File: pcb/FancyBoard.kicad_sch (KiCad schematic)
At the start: 179 parts, among them J1 Conn_01x02_Socket, SW1 SW_Push_45deg, SW10 SW_Push_45deg, SW11 SW_Push_45deg, SW12 SW_Push_45deg, SW13 SW_Push_45deg, SW14 SW_Push_45deg, SW15 SW_Push_45deg, SW16 SW_Push_45deg, SW17 SW_Push_45deg, SW18 SW_Push_45deg, SW19 SW_Push_45deg, SW2 SW_Push_45deg, SW20 SW_Push_45deg, SW21 SW_Push_45deg, SW22 SW_Push_45deg, SW23 SW_Push_45deg, SW24 SW_Push_45deg, SW25 SW_Push_45deg, SW26 SW_Push_45deg, SW27 SW_Push_45deg, SW28 SW_Push_45deg, SW29 SW_Push_45deg, SW3 SW_Push_45deg, SW30 SW_Push_45deg, SW31 SW_Push_45deg, SW32 SW_Push_45deg, SW33 SW_Push_45deg, SW34 SW_Push_45deg, SW35 SW_Push_45deg, SW36 SW_Push_45deg, SW37 SW_Push_45deg, SW38 SW_Push_45deg, SW39 SW_Push_45deg, SW4 SW_Push_45deg, SW40 SW_Push_45deg, SW41 SW_Push_45deg, SW42 SW_Push_45deg, SW43 SW_Push_45deg, SW44 SW_Push_45deg, SW45 SW_Push_45deg, SW46 SW_Push_45deg, SW47 SW_Push_45deg, SW48 SW_Push_45deg, SW49 SW_Push_45deg, SW5 SW_Push_45deg, SW50 SW_Push_45deg, SW51 SW_Push_45deg, SW52 SW_Push_45deg, SW53 SW_Push_45deg, SW54 SW_Push_45deg, SW55 SW_Push_45deg, SW56 SW_Push_45deg, SW57 SW_Push_45deg, SW58 SW_Push_45deg, SW59 SW_Push_45deg, SW6 SW_Push_45deg, SW60 SW_Push_45deg, SW61 SW_Push_45deg, SW62 SW_Push_45deg, SW63 SW_Push_45deg, SW64 SW_Push_45deg, SW65 SW_Push_45deg, SW66 SW_Push_45deg, SW67 SW_Push_45deg, SW68 SW_Push_45deg, SW69 SW_Push_45deg, SW7 SW_Push_45deg, SW70 SW_Push_45deg, SW71 SW_Push_45deg, SW72 SW_Push_45deg, SW73 SW_Push_45deg, SW74 SW_Push_45deg, SW75 SW_Push_45deg, SW76 SW_Push_45deg, SW77 SW_Push_45deg, SW78 SW_Push_45deg, SW8 SW_Push_45deg, SW9 SW_Push_45deg, SW93 RotaryEncoder_Switch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

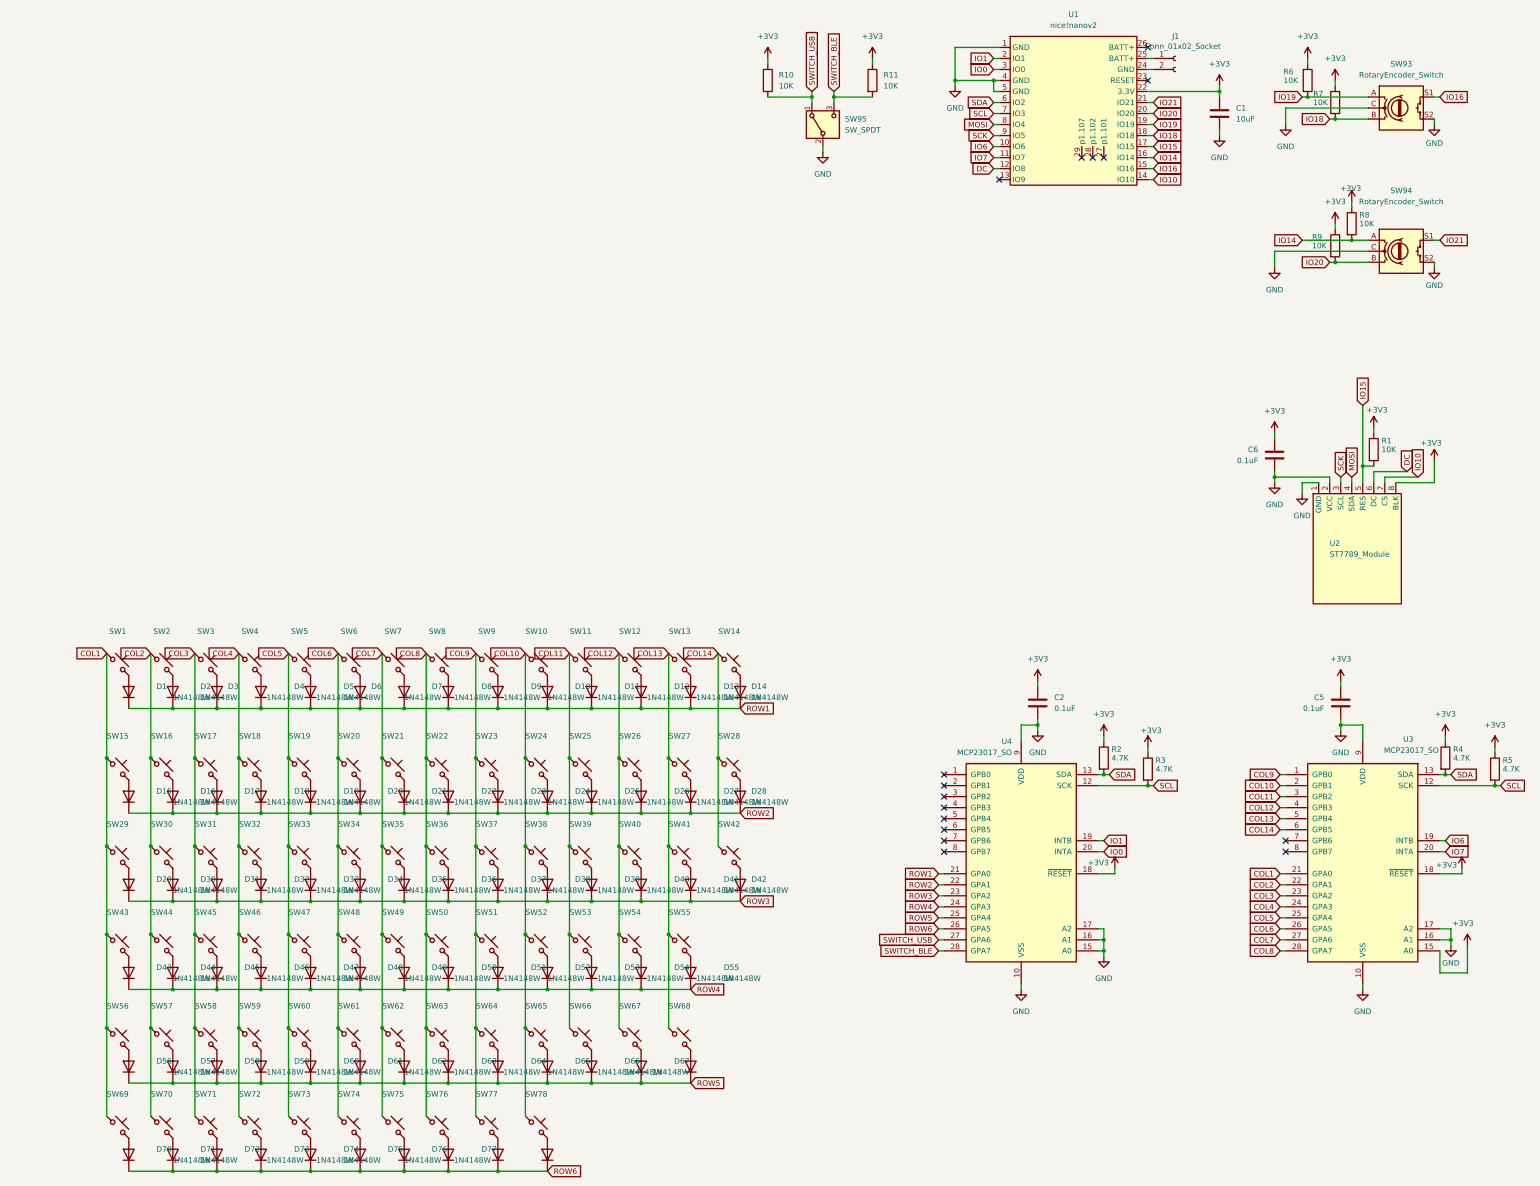
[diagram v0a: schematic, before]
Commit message: pcb done
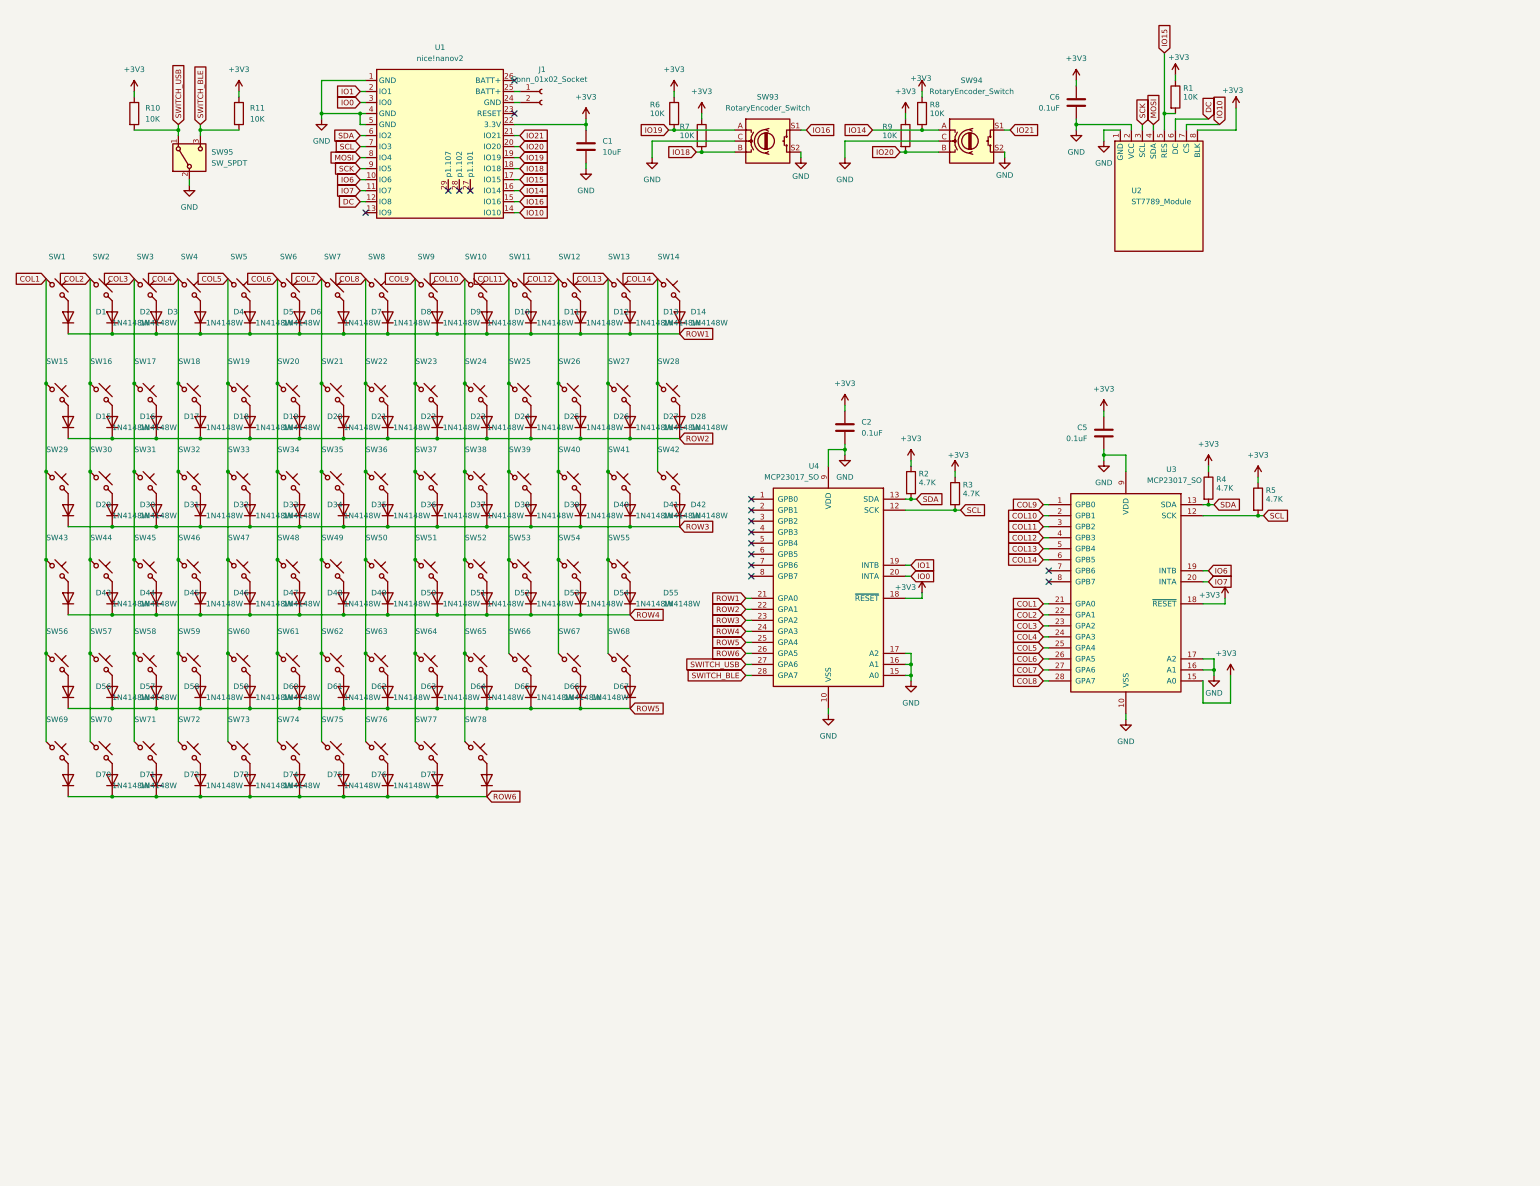
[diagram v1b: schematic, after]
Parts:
- SW95: footprint SS-12D00:SS12-D00 -> MSK-12C02:MSK-12C02
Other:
- moved on the sheet: C1, C2, C5, C6, D1, D10, D11, D12, D13, D14, D15, D16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
